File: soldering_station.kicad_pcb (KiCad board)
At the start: 2 copper layers, 70 parts, among them IC1 ATMEGA8A-P, P1 17v, P2 220v, P3 24v|220v, P4 solder, P5 thermocouple, P6 Fan, P7 thermocouple, P8 Heater, Q1 КТ313Б, Q2 КТ313Б, Q3 КТ313Б, Q4 КТ815А, SW1 mode, SW2 Enc, U1 TL072, U2 MOC3023M, U3 MOC3023M, U4 LM7805CT

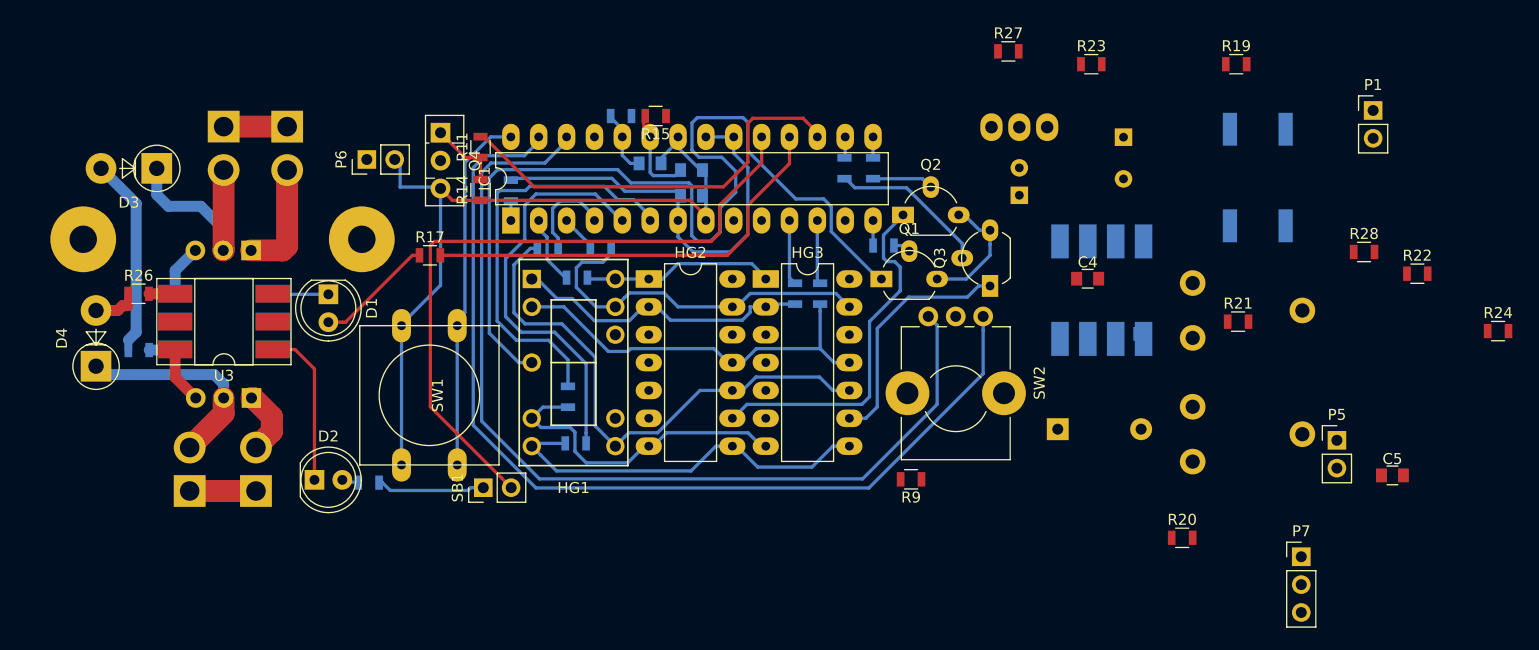
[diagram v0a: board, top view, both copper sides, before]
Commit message: Fix
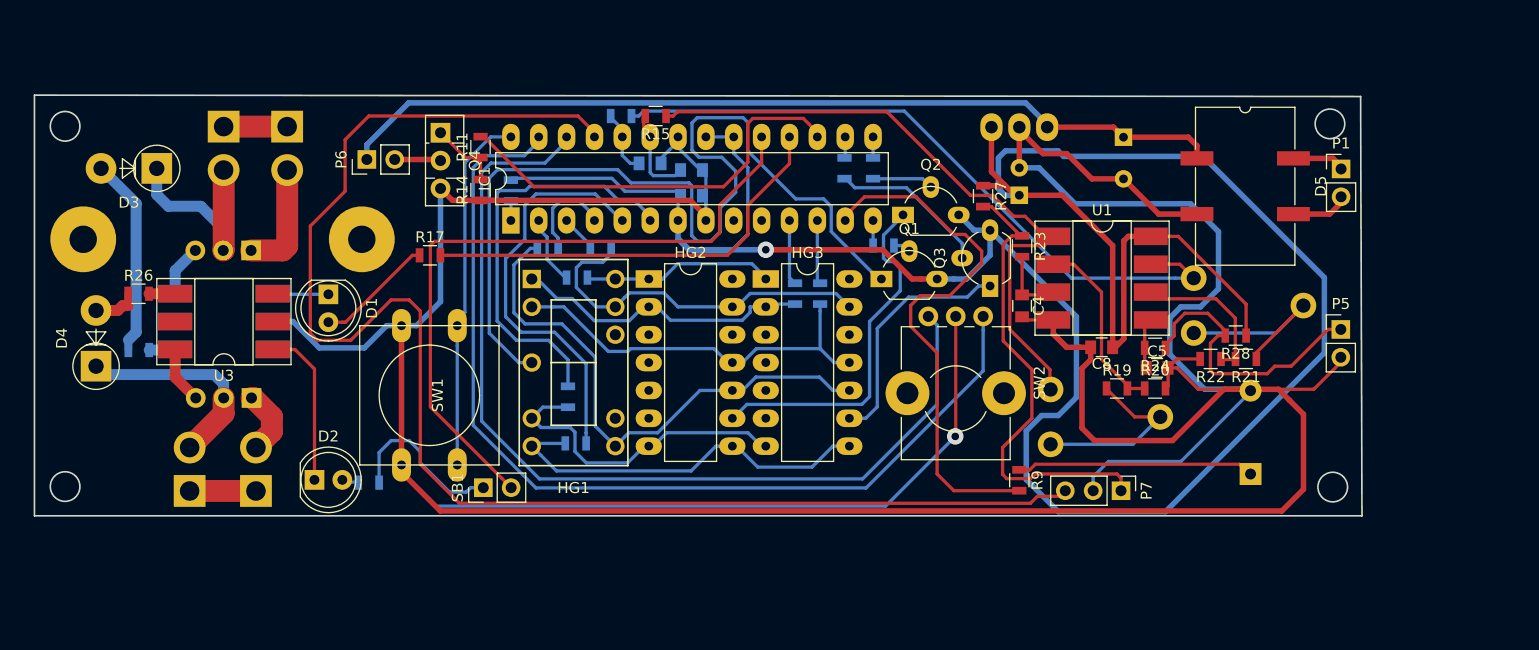
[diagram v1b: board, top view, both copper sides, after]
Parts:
- C8, D5, U1: moved to F.Cu
- moved R19 31.5 mm to (159.5, 68.5)
- moved R24 31.3 mm to (163.0, 64.8), turned to 180 degrees
- moved C5 23.6 mm to (163.2, 66.6)
- moved R22 20.4 mm to (168.1, 65.8), turned to 180 degrees
- moved BZ1 18.0 mm to (171.7, 76.3), turned to 90 degrees
- moved R23 17.8 mm to (150.9, 55.6), turned to 270 degrees
- moved P7 17.5 mm to (159.9, 77.9), turned to 270 degrees
- moved R28 14.0 mm to (170.3, 63.7), turned to 180 degrees
- moved R20 13.8 mm to (163.0, 68.5)
- moved R27 13.4 mm to (147.3, 51.0), turned to 270 degrees
- moved RV1 13.0 mm to (153.5, 68.6)
- moved P5 10.1 mm to (179.9, 63.1)
- moved R9 9.87 mm to (150.6, 76.9), turned to 270 degrees
- moved C4 6.47 mm to (150.9, 61.0), turned to 270 degrees
- moved P1 6.08 mm to (180.0, 48.5)
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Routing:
- net GND: track 70.3 -> 389.0 mm, vias 0 -> 1
- net +5V: track 51.3 -> 244.0 mm, vias 0 -> 1
- net Net-(IC1-Pad25): track 7.88 -> 130.6 mm
- net +24V: track 0.00 -> 81.5 mm
- net Net-(P2-Pad1): track 75.4 -> 5.79 mm
- net Net-(R16-Pad1): track 0.00 -> 62.2 mm
- net Net-(R15-Pad1): track 0.00 -> 59.8 mm
- net Net-(HG1-Pad4): track 30.1 -> 86.0 mm
- net Net-(IC1-Pad13): track 0.00 -> 49.3 mm
- net Net-(P7-Pad1): track 3.79 -> 42.7 mm
- net Net-(P5-Pad1): track 0.00 -> 27.0 mm
- net Net-(BZ1-Pad1): track 0.00 -> 21.7 mm
- net Net-(R19-Pad1): track 0.00 -> 17.9 mm
- net Net-(R21-Pad1): track 0.00 -> 17.7 mm
- net Net-(R19-Pad2): track 0.00 -> 16.8 mm
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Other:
- board outline added: 121 x 38.4 mm

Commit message: Add 3D view
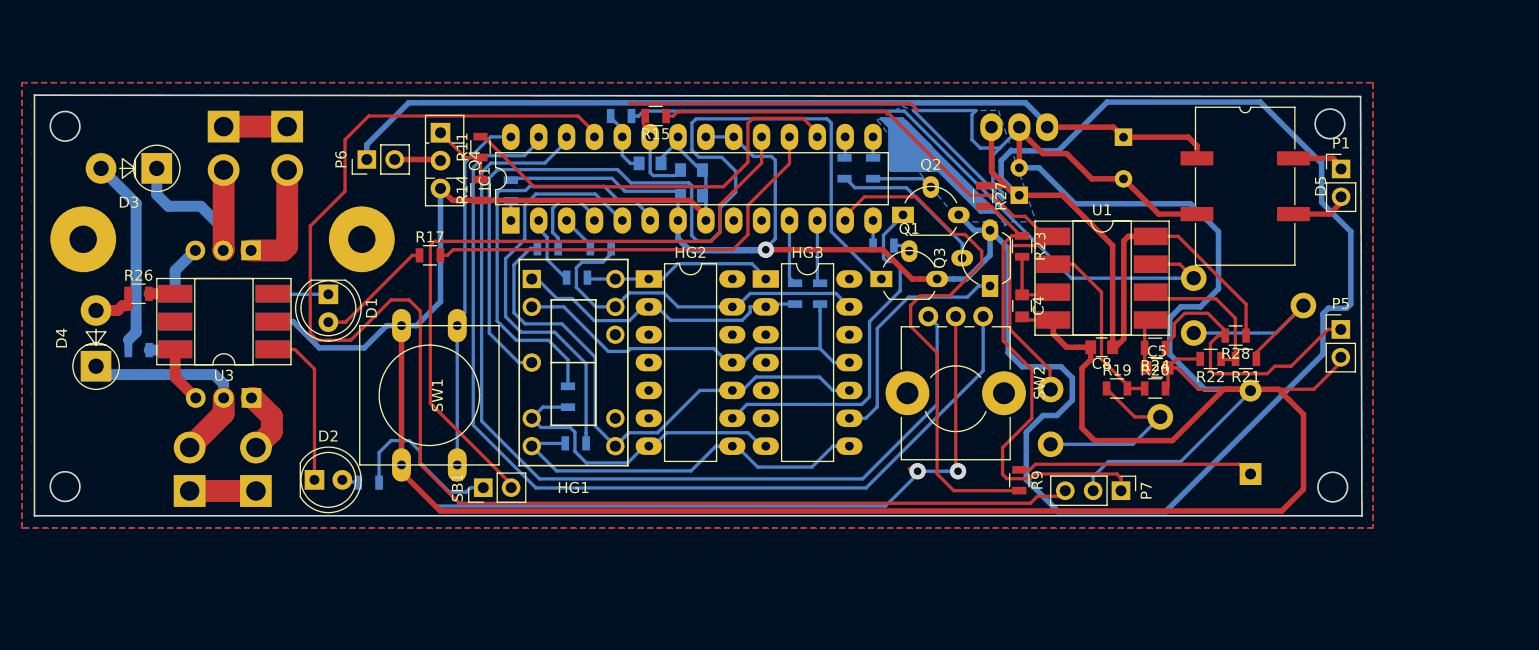
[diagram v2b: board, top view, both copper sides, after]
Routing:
- net (no net): track 0.00 -> 81.5 mm
- net GND: track 389.0 -> 423.3 mm, vias 1 -> 2
- net +5V: track 244.0 -> 261.8 mm
- net Net-(HG1-Pad4): track 86.0 -> 88.9 mm
- added copper zone on B.Cu, net GND
- added copper zone on F.Cu, net GND
